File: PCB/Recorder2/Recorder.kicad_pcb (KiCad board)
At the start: 2 copper layers, 70 x 70 mm, 57 parts, among them J1 Reset, J3 TC2030-USB-NL-DS, J4 TF_PUSH, J5 USB-C-Socket-H, J6 Battery, Q1 CJ2301, SW1 SW_Push_DPDT, U1 ESP32-S3-MINI-1-N4R2, U2 TPS22916CNYFPR, U3 TP4054, U4 ME6211C33M5G-N, U5 ICS-43434, U6 ICS-43434

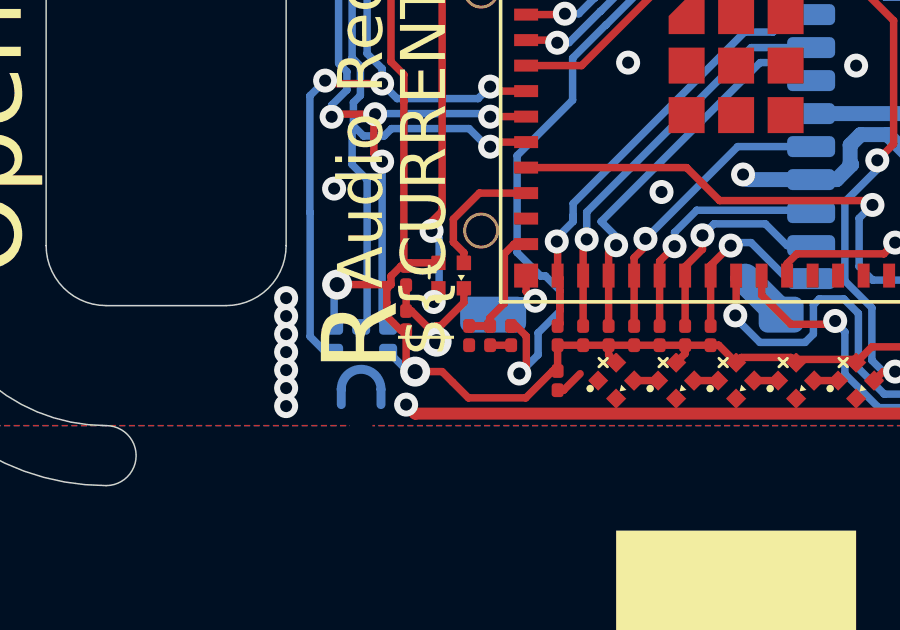
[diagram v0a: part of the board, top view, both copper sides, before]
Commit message: Twqeak
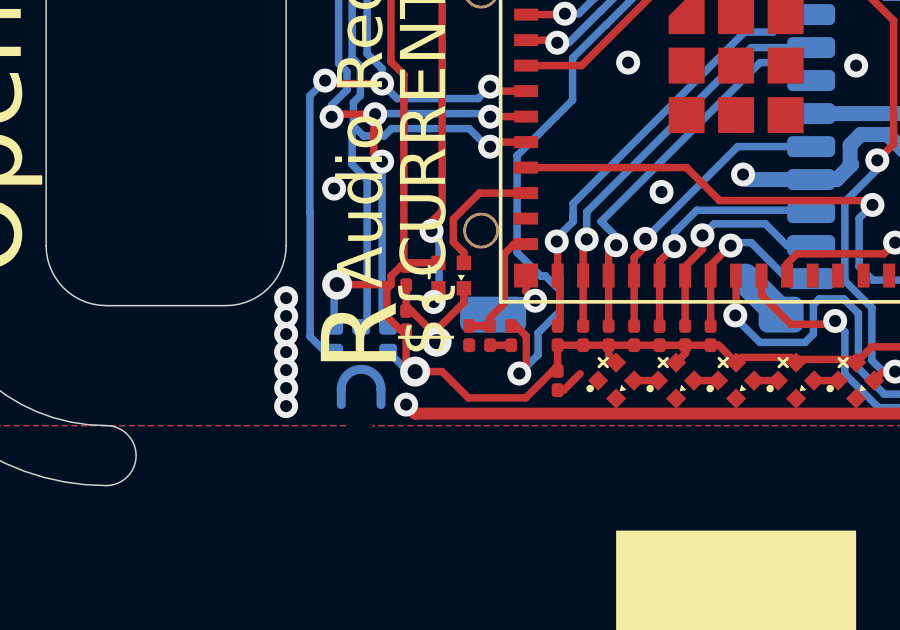
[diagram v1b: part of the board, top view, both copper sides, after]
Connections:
- SW1 pad 1: GND -> unconnected-(SW1-A-Pad1)

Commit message: beep bug
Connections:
- net VBAT renamed VBATCHG
